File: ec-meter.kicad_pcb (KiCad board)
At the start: 2 copper layers, 47 x 57 mm, 39 parts, among them P1 Probe, P2 V+, P3 OUT, P4 V-, U1 LM324, U2 LM324

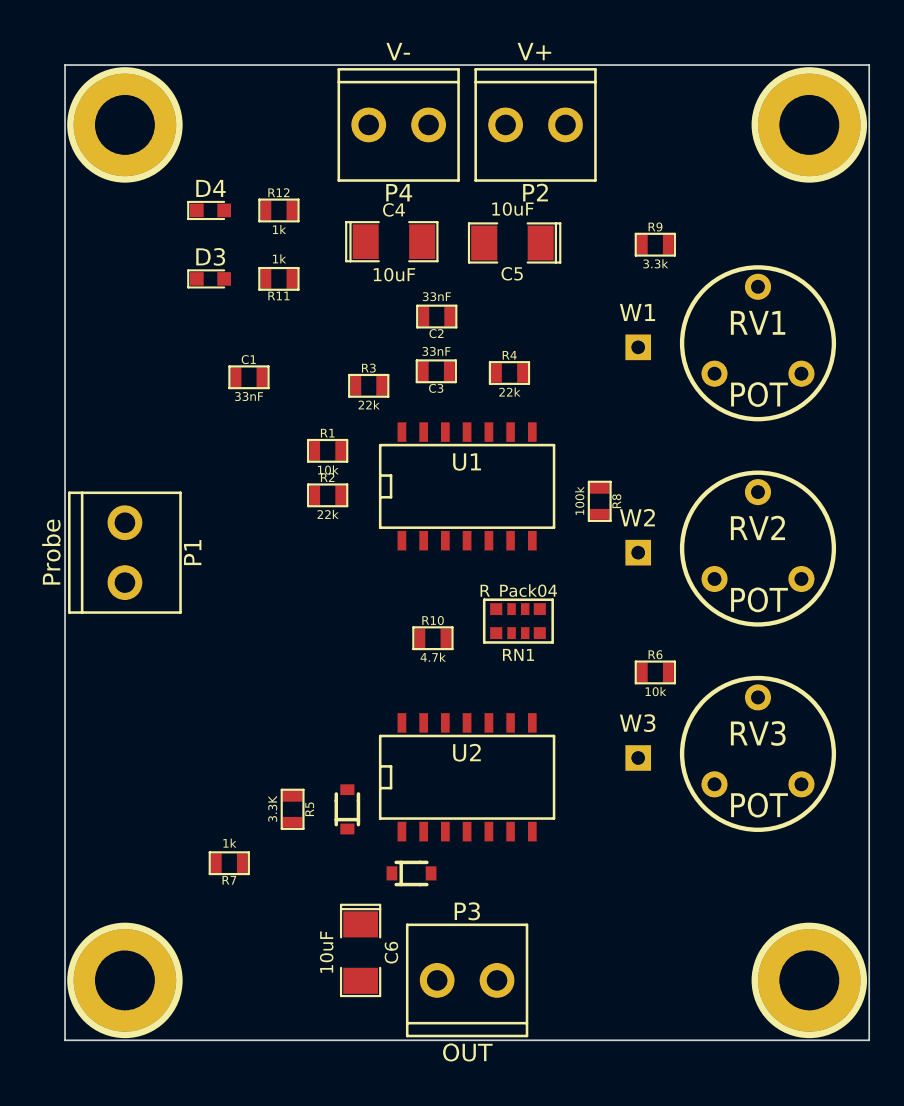
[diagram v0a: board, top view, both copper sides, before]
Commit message: Did routing
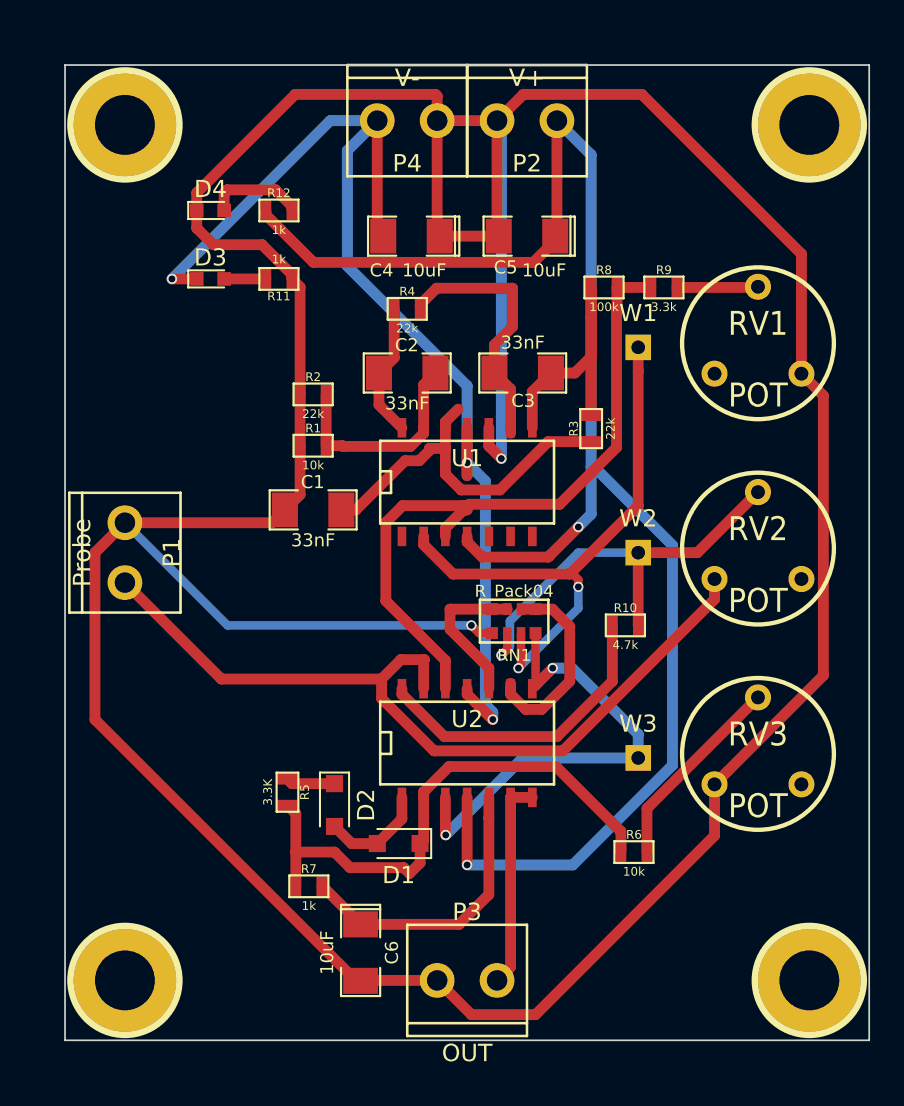
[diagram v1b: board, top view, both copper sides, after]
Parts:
- C1, C2, C3: footprint visgence_parts:SM0603_VIS -> visgence_parts:SM1206_VIS
- D1, D2: footprint visgence_parts:SOD-323 -> Diodes_SMD:D_SOD-323_HandSoldering
- moved R3 13.2 mm to (57.2, 42.8), turned to 90 degrees
- moved R8 12.5 mm to (58.0, 34.5), turned to 0 degrees
- moved R10 11.3 mm to (59.2, 54.2)
- moved R6 10.6 mm to (59.8, 67.5)
- moved C1 8.61 mm to (41.0, 47.5)
- moved R4 7.05 mm to (46.5, 35.8)
- moved R2 5.96 mm to (41.0, 40.8)
- moved C3 5.05 mm to (53.2, 39.5)
- moved R7 4.84 mm to (40.8, 69.5), turned to 0 degrees
- moved C2 3.72 mm to (46.5, 39.5), turned to 0 degrees
- moved R9 2.55 mm to (61.5, 34.5)
- moved U2 2.00 mm to (50.0, 61.0)
- moved D1 1.90 mm to (46.0, 67.0)
- moved C4 1.08 mm to (46.8, 31.5), turned to 180 degrees
- moved R5 1.04 mm to (39.5, 64.0)
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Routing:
- net GND: track 0.00 -> 236.7 mm, vias 0 -> 2
- net +5V: track 0.00 -> 96.6 mm, vias 0 -> 2
- net -5V: track 0.00 -> 69.4 mm, vias 0 -> 3
- net Probe: track 0.00 -> 48.7 mm
- net Net-(R8-Pad2): track 0.00 -> 40.4 mm
- net SineOut: track 0.00 -> 34.0 mm, vias 0 -> 2
- net Net-(D1-Pad1): track 0.00 -> 32.1 mm
- net Diffout: track 0.00 -> 28.1 mm, vias 0 -> 2
- net AmpOut: track 0.00 -> 25.5 mm, vias 0 -> 1
- net Net-(C1-Pad2): track 0.00 -> 22.1 mm
- net Net-(R10-Pad1): track 0.00 -> 18.2 mm
- net Net-(C3-Pad1): track 0.00 -> 17.9 mm
- net Net-(C6-Pad1): track 0.00 -> 17.1 mm
- net Net-(C3-Pad2): track 0.00 -> 15.3 mm
- net Net-(C2-Pad2): track 0.00 -> 12.8 mm
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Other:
- net class Default: trace_width 0.25 -> 0.635
